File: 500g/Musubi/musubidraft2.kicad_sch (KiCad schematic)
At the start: 28 parts, among them IC2 DRV8212DRLR, IC3 DRV8212DRLR, J1 BDC1, J2 BDC2, J2 LINE_SENS1, J3 LINE_SENS2, J4 DDS1, J4 LIDAR2, J5 DDS2, J9 Battery, U1 DEV-16771, U2 LM2576S-5, U3 LM2576-3.3WT

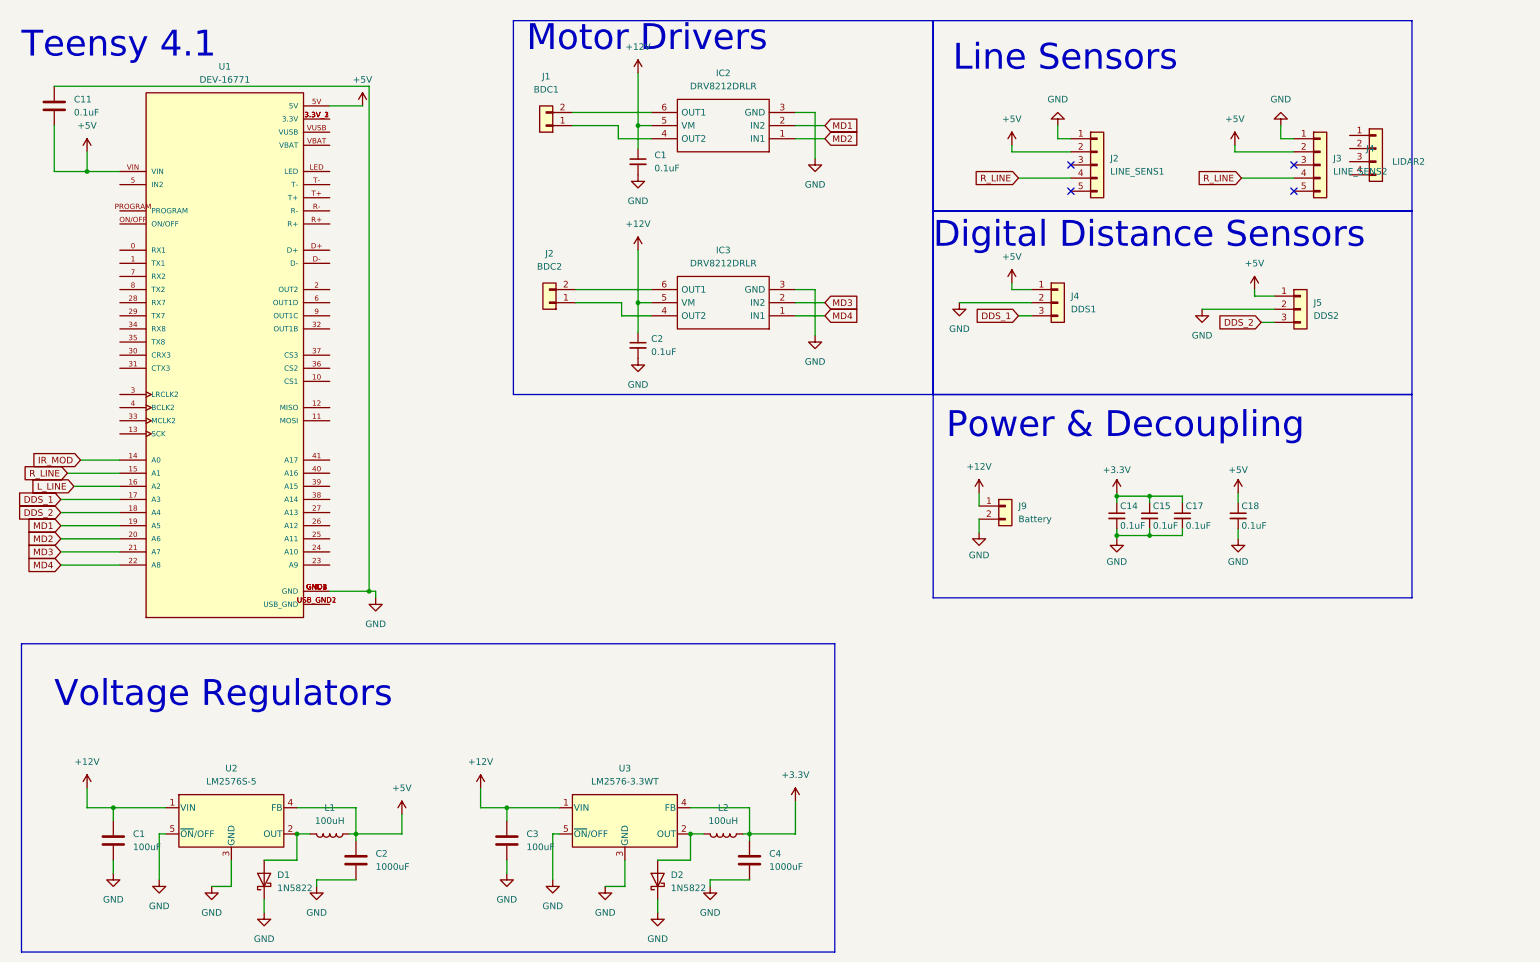
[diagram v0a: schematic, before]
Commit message: added sensors bc papa alex said so
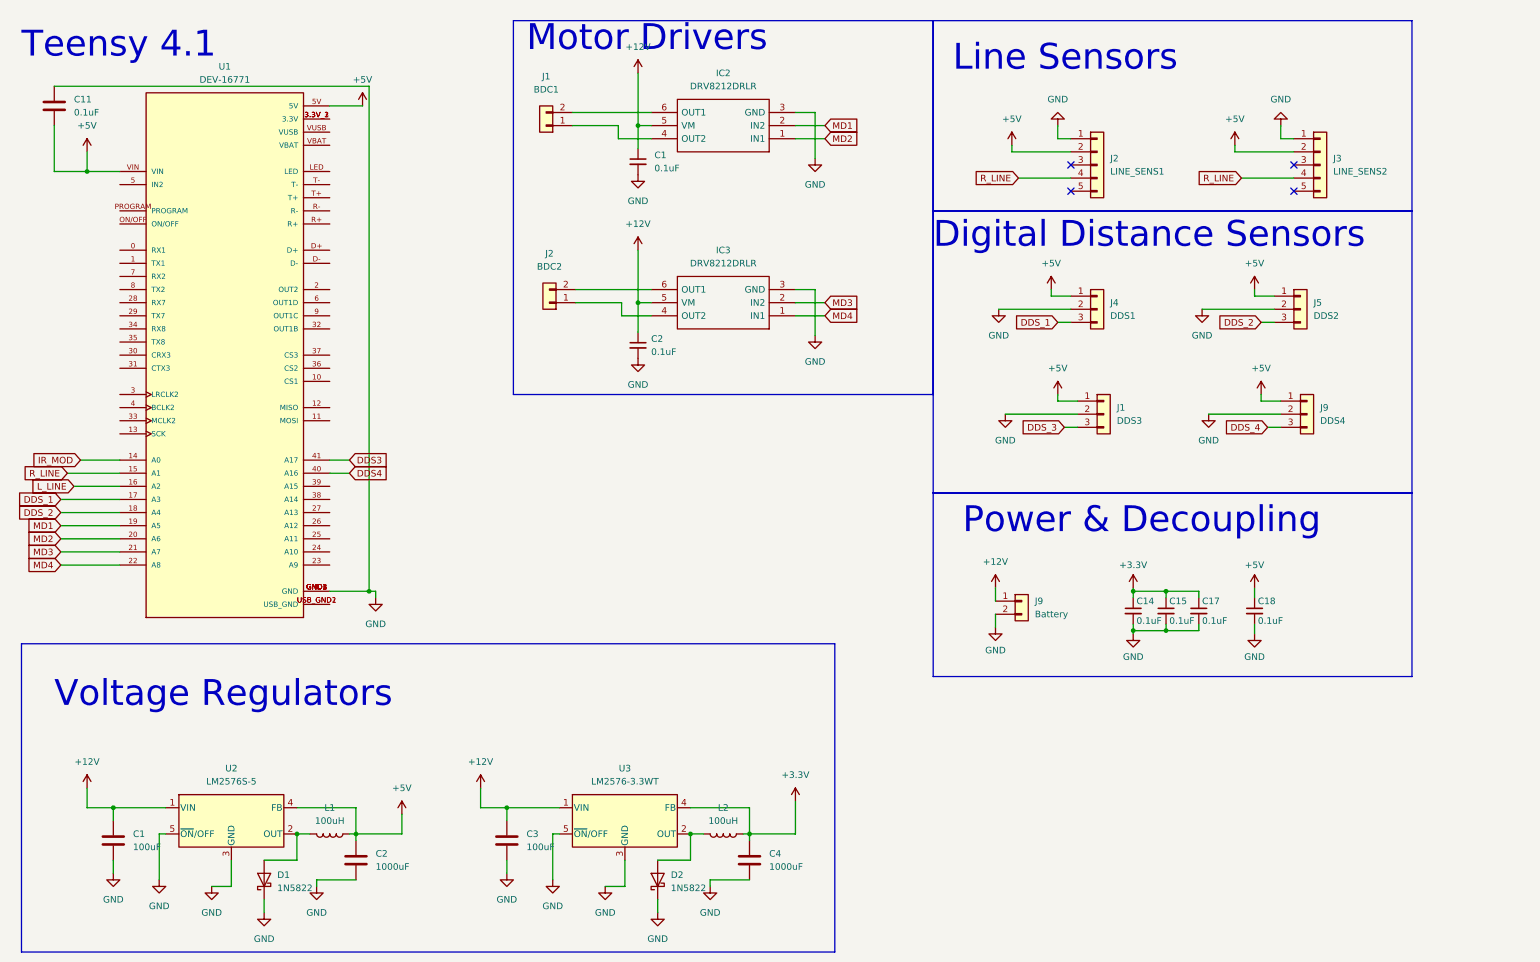
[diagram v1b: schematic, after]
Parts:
- removed J4: LIDAR2, symbol Connector_Generic:Conn_01x04
- added J1: DDS3, symbol Connector_Generic:Conn_01x03
- added J9: DDS4, symbol Connector_Generic:Conn_01x03
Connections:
- net +5V: now also J1.1 (Pin_1), J9.1 (Pin_1)
- net GND: now also J1.2 (Pin_2), J9.2 (Pin_2)
- net DDS4: now reaches U1.40 (A16)
- net DDS3: now reaches U1.41 (A17)
- new net DDS_3: J1.3 (Pin_3)
- new net DDS_4: J9.3 (Pin_3)
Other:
- moved on the sheet: C14, C15, C17, C18, J4, J9
